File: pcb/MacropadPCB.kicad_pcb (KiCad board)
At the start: 2 copper layers, 73 x 73 mm, 27 parts, among them J1 Conn_01x04_Pin, SW1 SW_Push_45deg, SW2 SW_Push_45deg, SW3 SW_Push_45deg, SW4 SW_Push_45deg, SW5 SW_Push_45deg, SW6 SW_Push_45deg, U1 MOUDLE-SEEEDUINO-XIAO

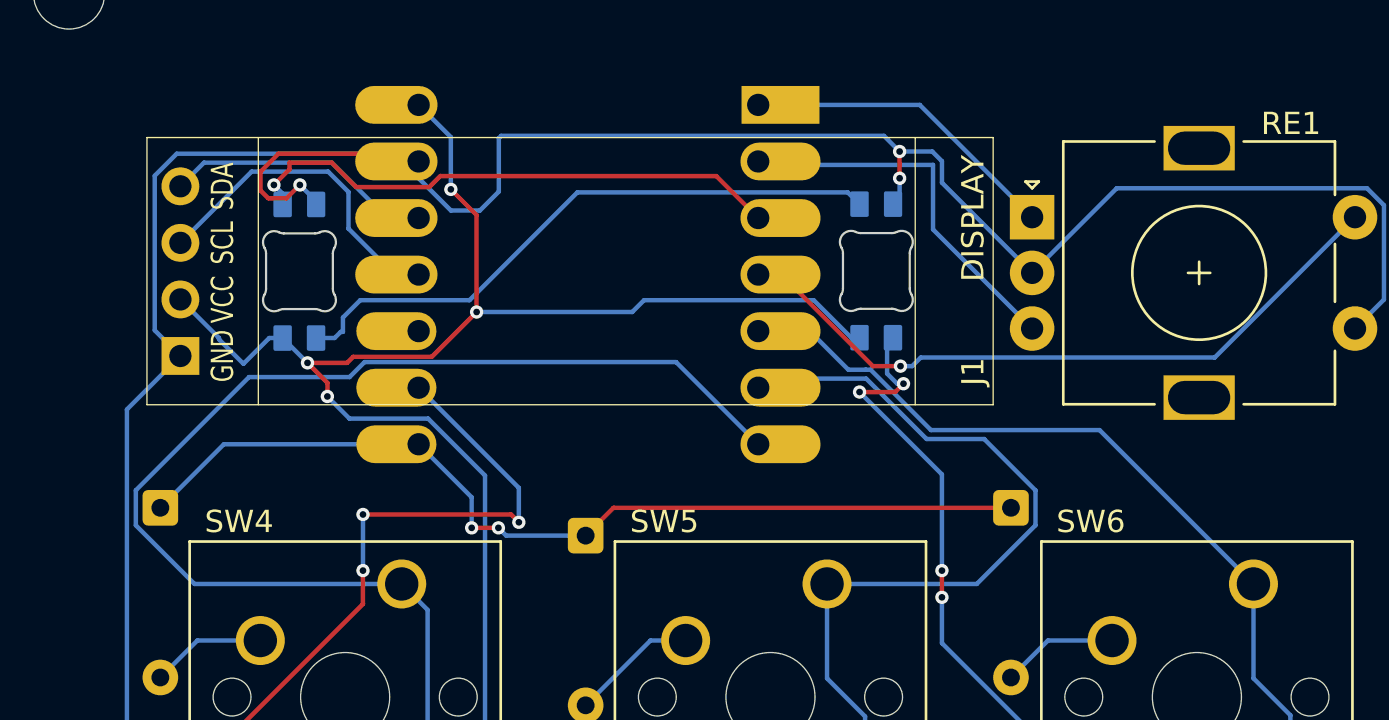
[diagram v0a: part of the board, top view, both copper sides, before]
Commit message: Update project images and final documentation refinements
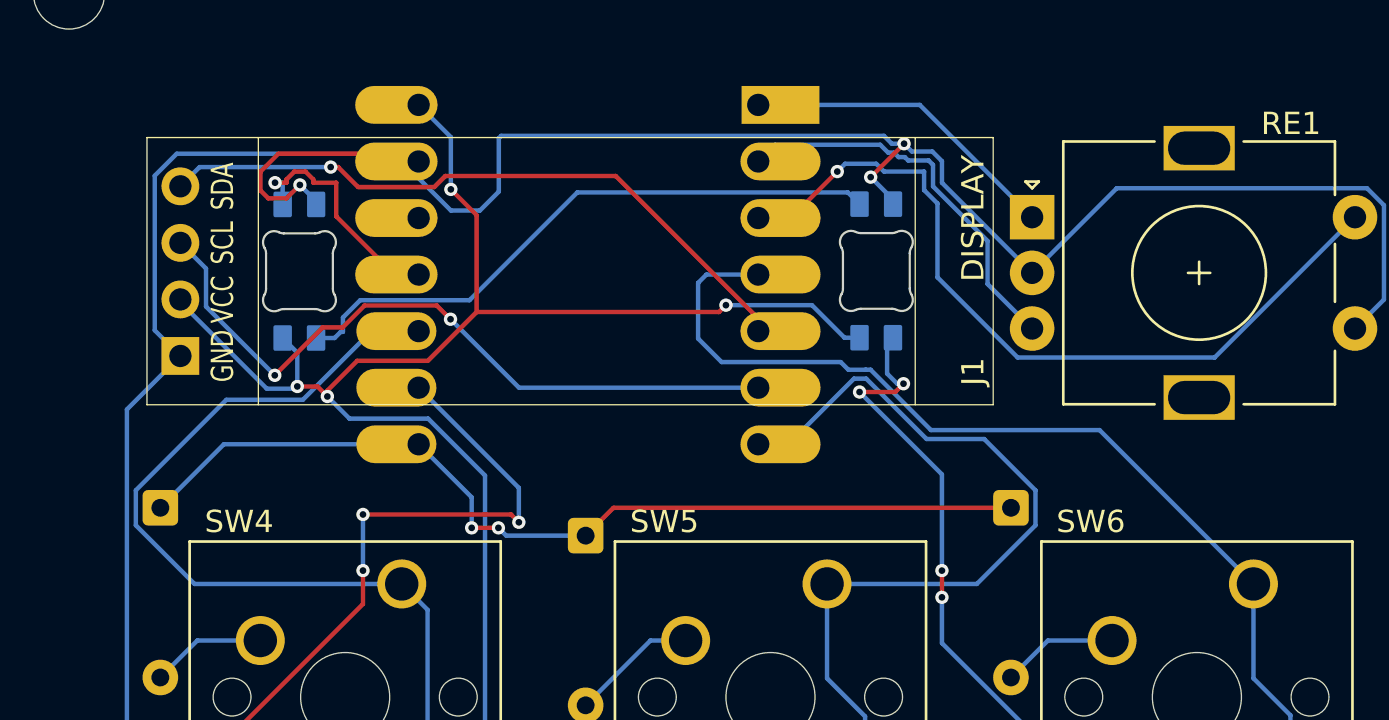
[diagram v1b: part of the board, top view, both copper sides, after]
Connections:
- U1 pad 10: unconnected-(U1-PA5_A9_D9_MISO-Pad10) -> COL0
- U1 pad 11: SCL -> SK_IN
- U1 pad 12: SDA -> unconnected-(U1-3V3-Pad12)
- U1 pad 3: SK_IN -> ENC_SW2
- U1 pad 4: ENC_SW2 -> COL2
- U1 pad 5: COL2 -> SDA
- U1 pad 6: COL1 -> SCL
- U1 pad 7: COL0 -> COL1
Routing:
- net SDA: track 12.2 -> 30.1 mm, vias 0 -> 1
- net SCL: track 14.9 -> 32.2 mm, vias 0 -> 2
- net SK_IN: track 27.4 -> 10.9 mm
- net COL0: track 66.7 -> 50.5 mm
- net COL2: track 47.8 -> 55.7 mm
- net ENC_SW2: track 31.3 -> 39.1 mm
- net GND: track 223.3 -> 224.6 mm
- net COL1: track 47.7 -> 48.7 mm
- net +5V: track 180.1 -> 181.1 mm
- net ENC_B: track 17.1 -> 17.7 mm
